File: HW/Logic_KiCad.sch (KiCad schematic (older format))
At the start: 35 parts, among them Q10 Q_NMOS_GSD, Q11 Q_NMOS_GSD, Q3 Q_NMOS_GSD, SW1 SW_SPDT, SW13 SW_SPST, SW14 SW_SPST, SW15 SW_SPST, U1 ESP32-PICO-D4

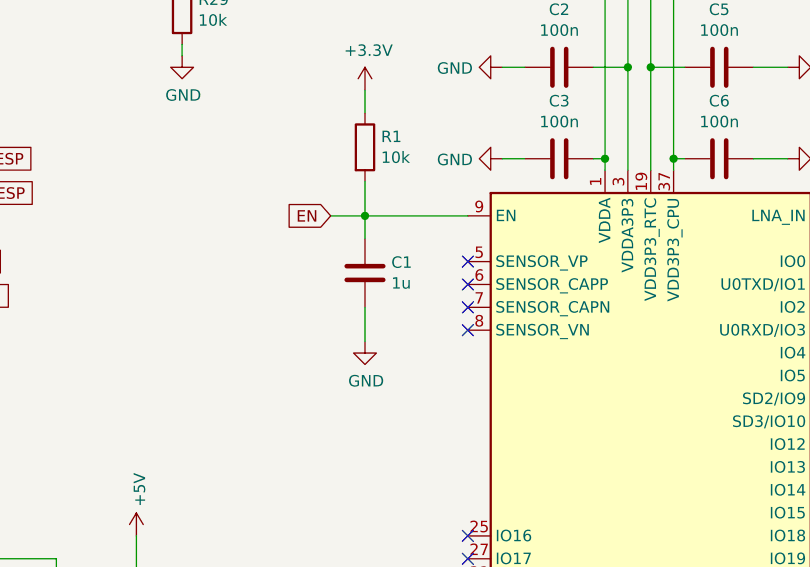
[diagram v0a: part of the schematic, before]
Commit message: Version 1.2 for fab
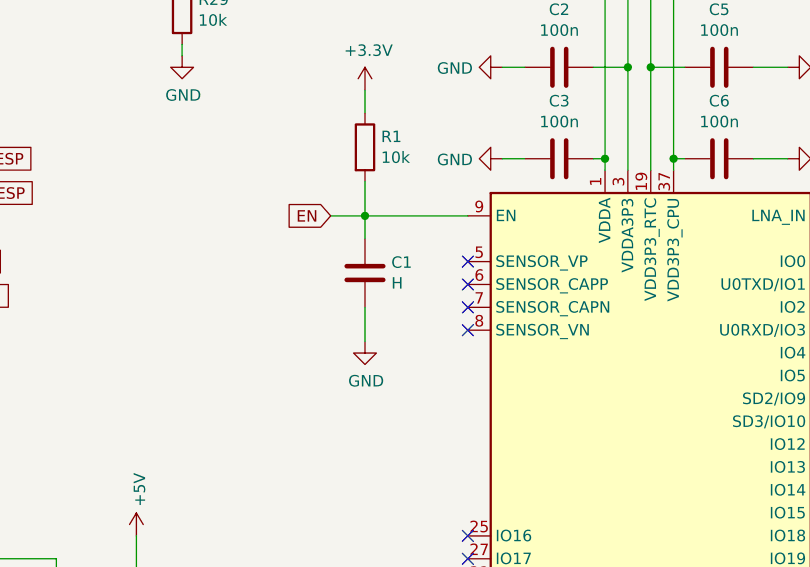
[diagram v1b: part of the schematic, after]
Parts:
- C1: value 1u -> H
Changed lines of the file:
@@
 P 3400 4500
 F 0 "C1" H 3285 4454 50  0000 R CNN
-F 1 "1u" H 3285 4545 50  0000 R CNN
+F 1 "H" H 3285 4545 50  0000 R CNN
 F 2 "Capacitor_SMD:C_0402_1005Metric" H 3438 4350 50  0001 C CNN
 F 3 "~" H 3400 4500 50  0001 C CNN
